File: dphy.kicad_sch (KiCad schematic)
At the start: 5 parts, among them J1002 FFC-22p-P0.5mm, U1002 RCLAMP0524P, U1003 RCLAMP0524P, U1004 RCLAMP0524P, U1005 RCLAMP0524P

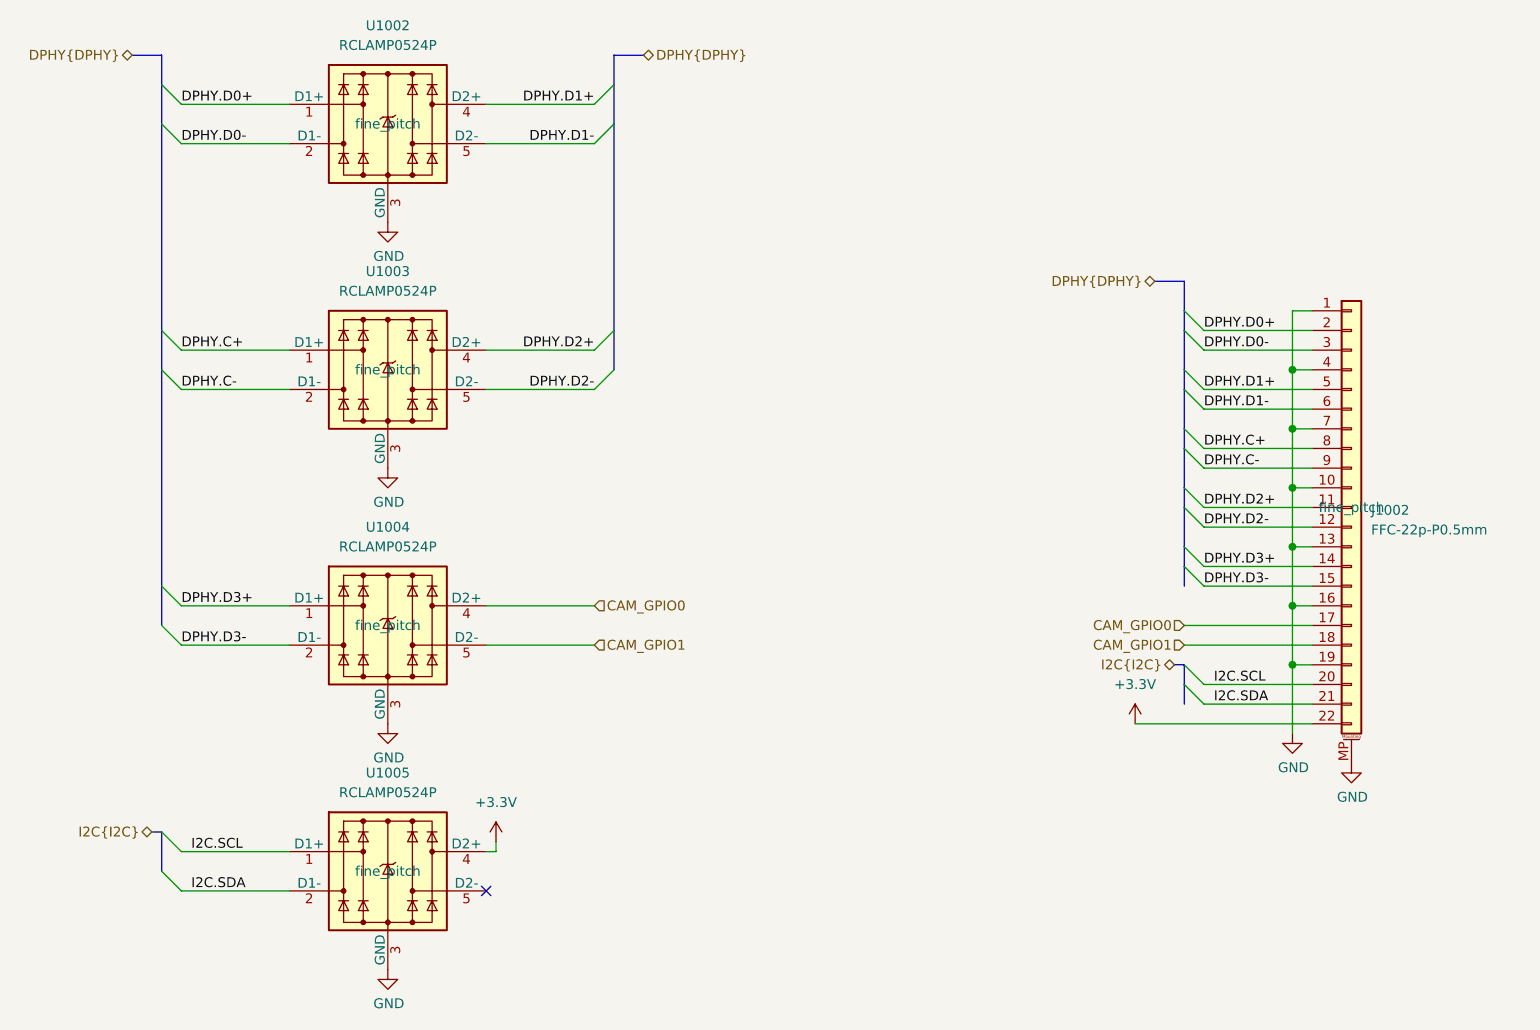
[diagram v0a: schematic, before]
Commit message: Fix schematic ERC errors
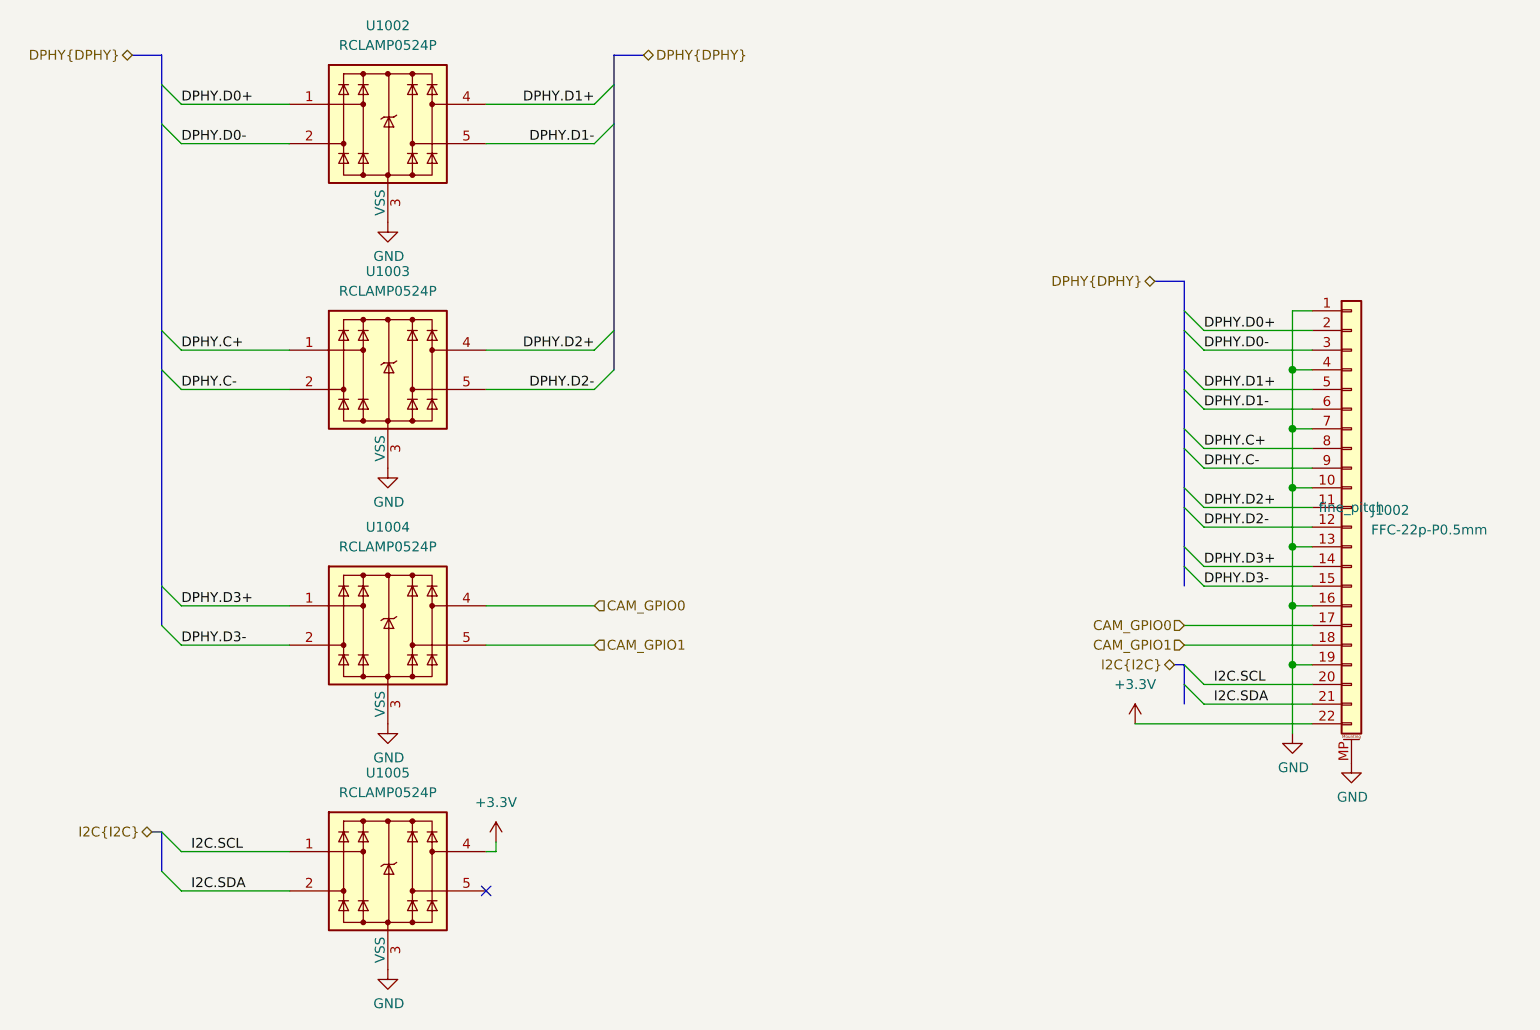
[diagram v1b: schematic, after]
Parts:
- U1002, U1003, U1004, U1005: footprint Package_SON:USON-10_2.5x1.0mm_P0.5mm -> Package_DFN_QFN:Diodes_UDFN-10_1.0x2.5mm_P0.5mm; symbol Yellow:TPD4EUSB30 -> Hatlabs:RCLAMP0524P
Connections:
- net +3.3V: no longer U1005.7 (D2+)
- net CAM_GPIO0: no longer U1004.7 (D2+)
- net CAM_GPIO1: no longer U1004.6 (D2-)
- net DPHY.C+: no longer U1003.10 (D1+)
- net DPHY.C-: no longer U1003.9 (D1-)
- net DPHY.D0+: no longer U1002.10 (D1+)
- net DPHY.D0-: no longer U1002.9 (D1-)
- net DPHY.D1+: no longer U1002.7 (D2+)
- net DPHY.D1-: no longer U1002.6 (D2-)
- net DPHY.D2+: no longer U1003.7 (D2+)
- net DPHY.D2-: no longer U1003.6 (D2-)
- net DPHY.D3+: no longer U1004.10 (D1+)
- net DPHY.D3-: no longer U1004.9 (D1-)
- net I2C.SCL: no longer U1005.10 (D1+)
- net I2C.SDA: no longer U1005.9 (D1-)
- net at U1005.5: no longer U1005.6 (D2-)
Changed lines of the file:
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@@
 	)
 	(symbol
-		(lib_name "Power_Protection:TPD4EUSB30_1")
-		(lib_id "Yellow:TPD4EUSB30")
+		(lib_id "Hatlabs:RCLAMP0524P")
 		(at 90.17 138.43 0)
 		(unit 1)
@@
 			)
 		)
-		(property "Footprint" "Package_SON:USON-10_2.5x1.0mm_P0.5mm"
+		(property "Footprint" "Package_DFN_QFN:Diodes_UDFN-10_1.0x2.5mm_P0.5mm"
 			(at 66.04 148.59 0)
 			(effects
@@
 			)
 		)
-		(property "Description" ""
+		(property "Description" "4-Channel Low Capacitance TVS Diode Array, DFN-10"
 			(at 90.17 138.43 0)
 			(effects
@@
 					(size 1.27 1.27)
 				)
-			)
-		)
-		(property "Sim.Enable" ""
-			(at 90.17 138.43 0)
-			(effects
-				(font
-					(size 1.27 1.27)
-				)
+				(hide yes)
 			)
 		)
@@
 	)
 	(symbol
-		(lib_name "Power_Protection:TPD4EUSB30_1")
-		(lib_id "Yellow:TPD4EUSB30")
+		(lib_id "Hatlabs:RCLAMP0524P")
 		(at 90.17 73.66 0)
 		(unit 1)
@@
 			)
 		)
-		(property "Footprint" "Package_SON:USON-10_2.5x1.0mm_P0.5mm"
+		(property "Footprint" "Package_DFN_QFN:Diodes_UDFN-10_1.0x2.5mm_P0.5mm"
 			(at 66.04 83.82 0)
 			(effects
@@
 			)
 		)
-		(property "Description" ""
+		(property "Description" "4-Channel Low Capacitance TVS Diode Array, DFN-10"
 			(at 90.17 73.66 0)
 			(effects
@@
 					(size 1.27 1.27)
 				)
-			)
-		)
-		(property "Sim.Enable" ""
-			(at 90.17 73.66 0)
-			(effects
-				(font
-					(size 1.27 1.27)
-				)
+				(hide yes)
 			)
 		)
@@
 	)
 	(symbol
-		(lib_name "Power_Protection:TPD4EUSB30_1")
-		(lib_id "Yellow:TPD4EUSB30")
+		(lib_id "Hatlabs:RCLAMP0524P")
 		(at 90.17 41.91 0)
 		(unit 1)
@@
 			)
 		)
-		(property "Footprint" "Package_SON:USON-10_2.5x1.0mm_P0.5mm"
+		(property "Footprint" "Package_DFN_QFN:Diodes_UDFN-10_1.0x2.5mm_P0.5mm"
 			(at 66.04 52.07 0)
 			(effects
@@
 			)
 		)
-		(property "Description" ""
+		(property "Description" "4-Channel Low Capacitance TVS Diode Array, DFN-10"
 			(at 90.17 41.91 0)
 			(effects
@@
 					(size 1.27 1.27)
 				)
-			)
-		)
-		(property "Sim.Enable" ""
-			(at 90.17 41.91 0)
-			(effects
-				(font
-					(size 1.27 1.27)
-				)
+				(hide yes)
 			)
 		)
@@
 			)
 		)
-		(property "Sim.Enable" ""
-			(at 214.63 91.44 0)
-			(effects
-				(font
-					(size 1.27 1.27)
-				)
-			)
-		)
 		(pin "1"
 		)
@@
 	)
 	(symbol
-		(lib_name "Power_Protection:TPD4EUSB30_1")
-		(lib_id "Yellow:TPD4EUSB30")
+		(lib_id "Hatlabs:RCLAMP0524P")
 		(at 90.17 106.68 0)
 		(unit 1)
@@
 			)
 		)
-		(property "Footprint" "Package_SON:USON-10_2.5x1.0mm_P0.5mm"
+		(property "Footprint" "Package_DFN_QFN:Diodes_UDFN-10_1.0x2.5mm_P0.5mm"
 			(at 66.04 116.84 0)
 			(effects
@@
 			)
 		)
-		(property "Description" ""
+		(property "Description" "4-Channel Low Capacitance TVS Diode Array, DFN-10"
 			(at 90.17 106.68 0)
 			(effects
@@
 					(size 1.27 1.27)
 				)
-			)
-		)
-		(property "Sim.Enable" ""
-			(at 90.17 106.68 0)
-			(effects
-				(font
-					(size 1.27 1.27)
-				)
-			)
-		)
+				(hide yes)
+			)
+		)
